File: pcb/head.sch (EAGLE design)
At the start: 9 parts

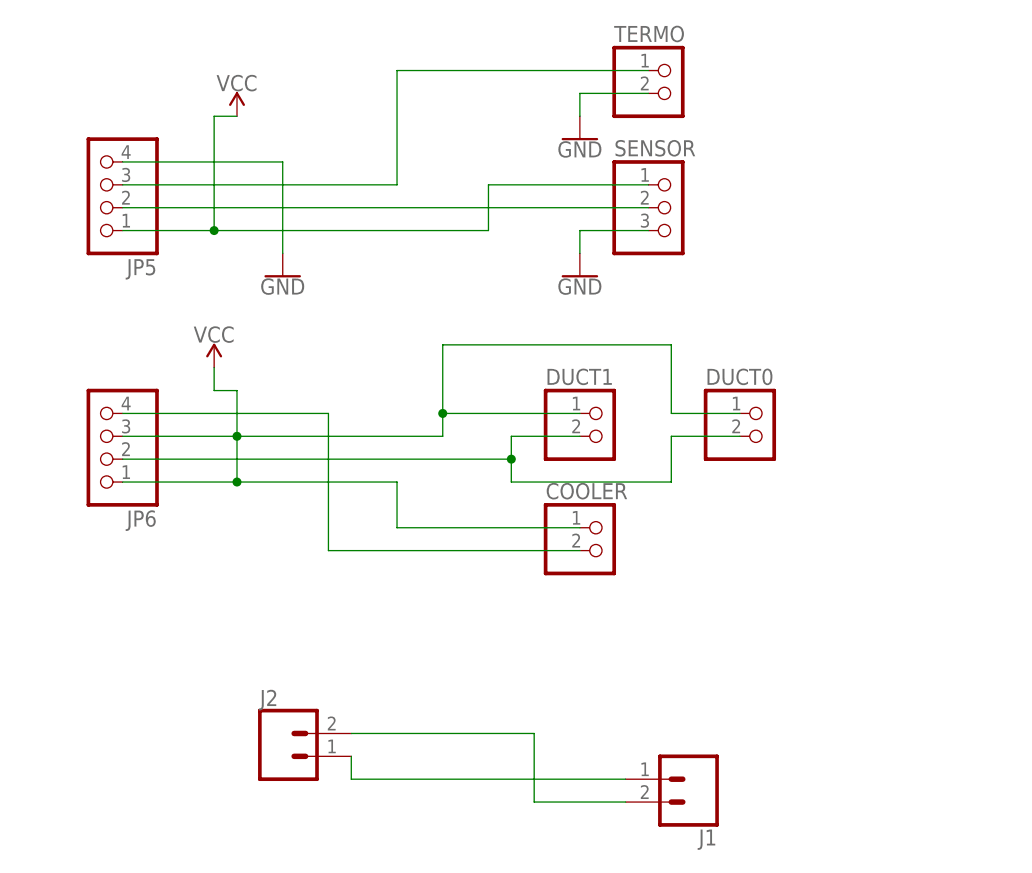
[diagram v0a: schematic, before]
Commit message: pcb
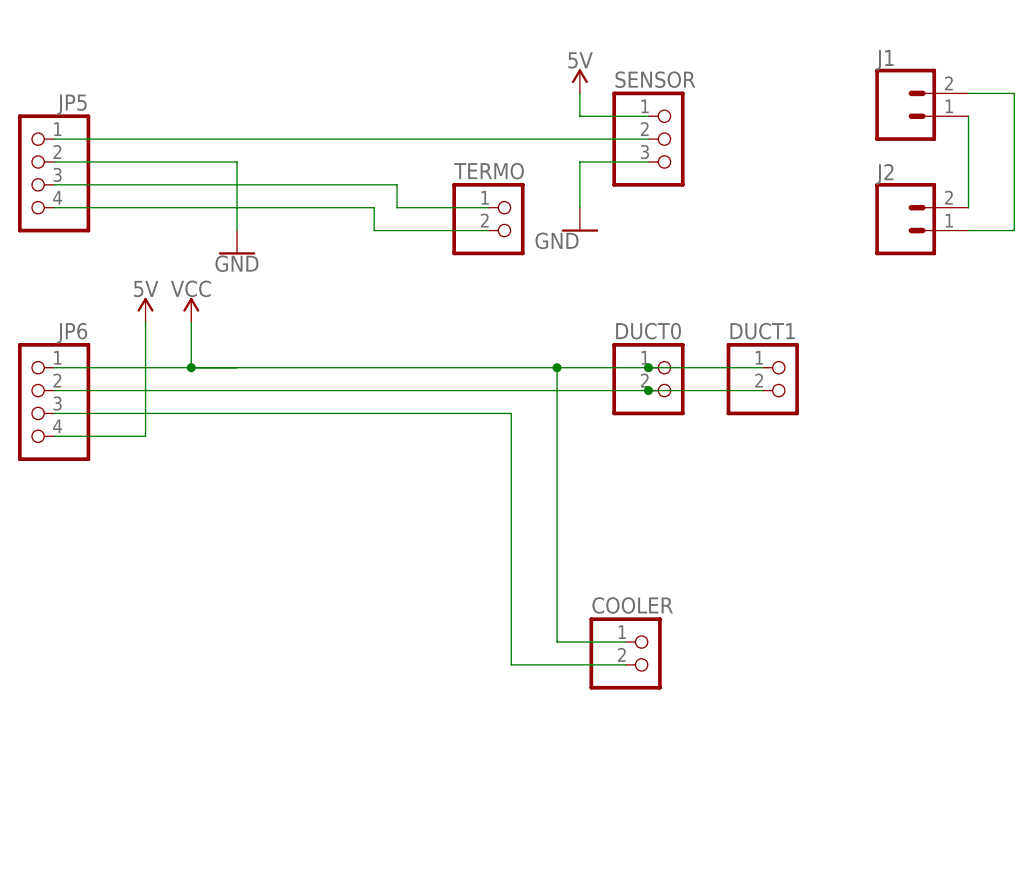
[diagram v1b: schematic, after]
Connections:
- new net 5V: JP6.4, SENSOR.1
- new net N$4: J1.1, J2.2
- net GND: now also JP5.2; no longer JP5.4, TERMO.2
- net N$1: now also JP5.1, SENSOR.2; no longer J1.1, J2.1
- net N$2: now also COOLER.2, JP6.3; no longer J1.2, J2.2
- net N$5: now also JP5.4, TERMO.2; no longer COOLER.2, JP6.4
- net N$6: now also J1.2, J2.1; no longer JP5.2, SENSOR.2
- net VCC: no longer JP5.1, JP6.3, SENSOR.1
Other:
- moved on the sheet: COOLER, DUCT0, DUCT1, J1, J2, JP5, JP6, SENSOR, TERMO
